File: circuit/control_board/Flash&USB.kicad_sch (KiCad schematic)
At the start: 4 parts, among them P1 USB_C_Plug_USB2.0, U13 CH440R, U14 MKDV1GCL-AB

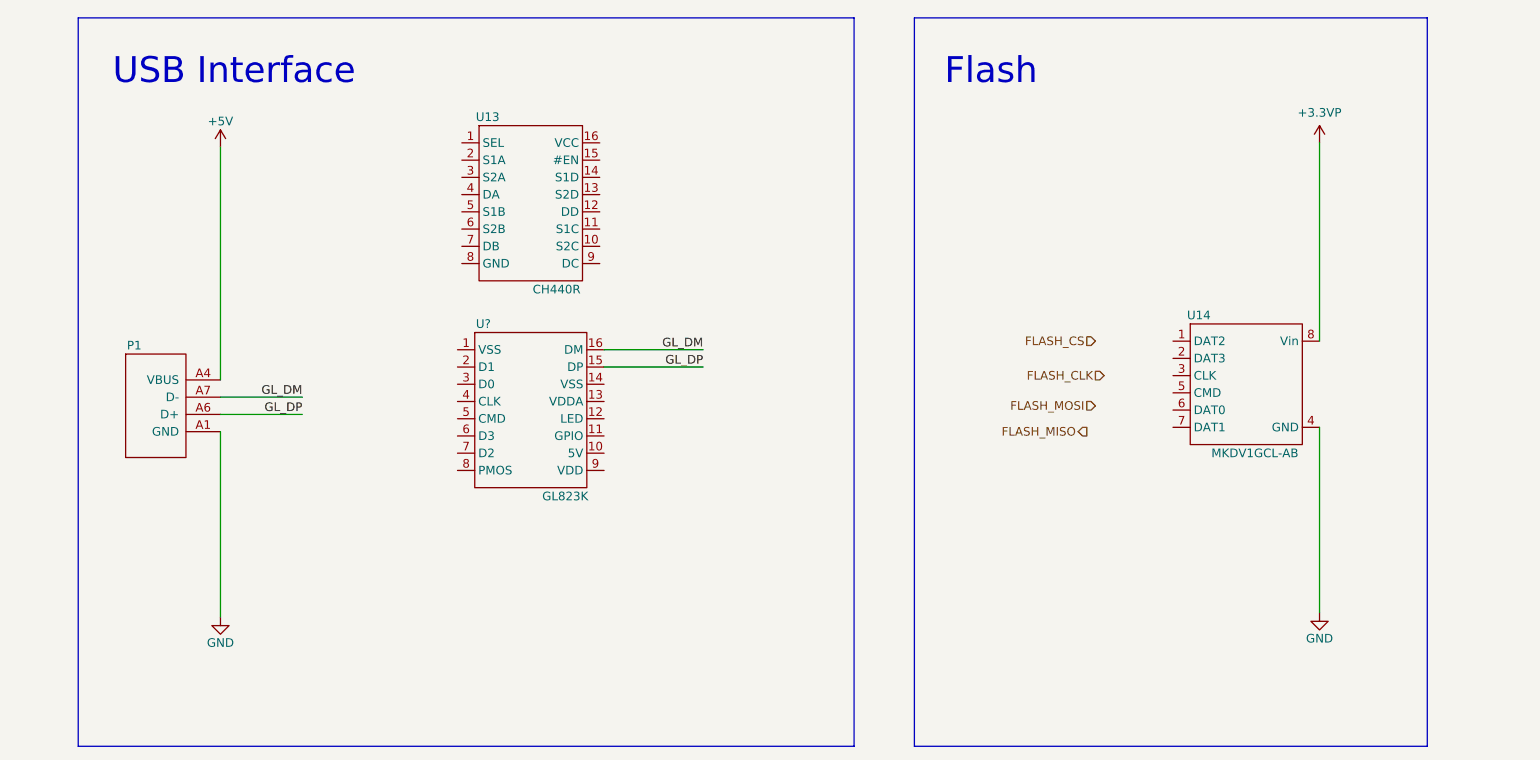
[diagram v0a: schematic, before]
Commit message: Update the main control board schematic to complete the SD card reader part.
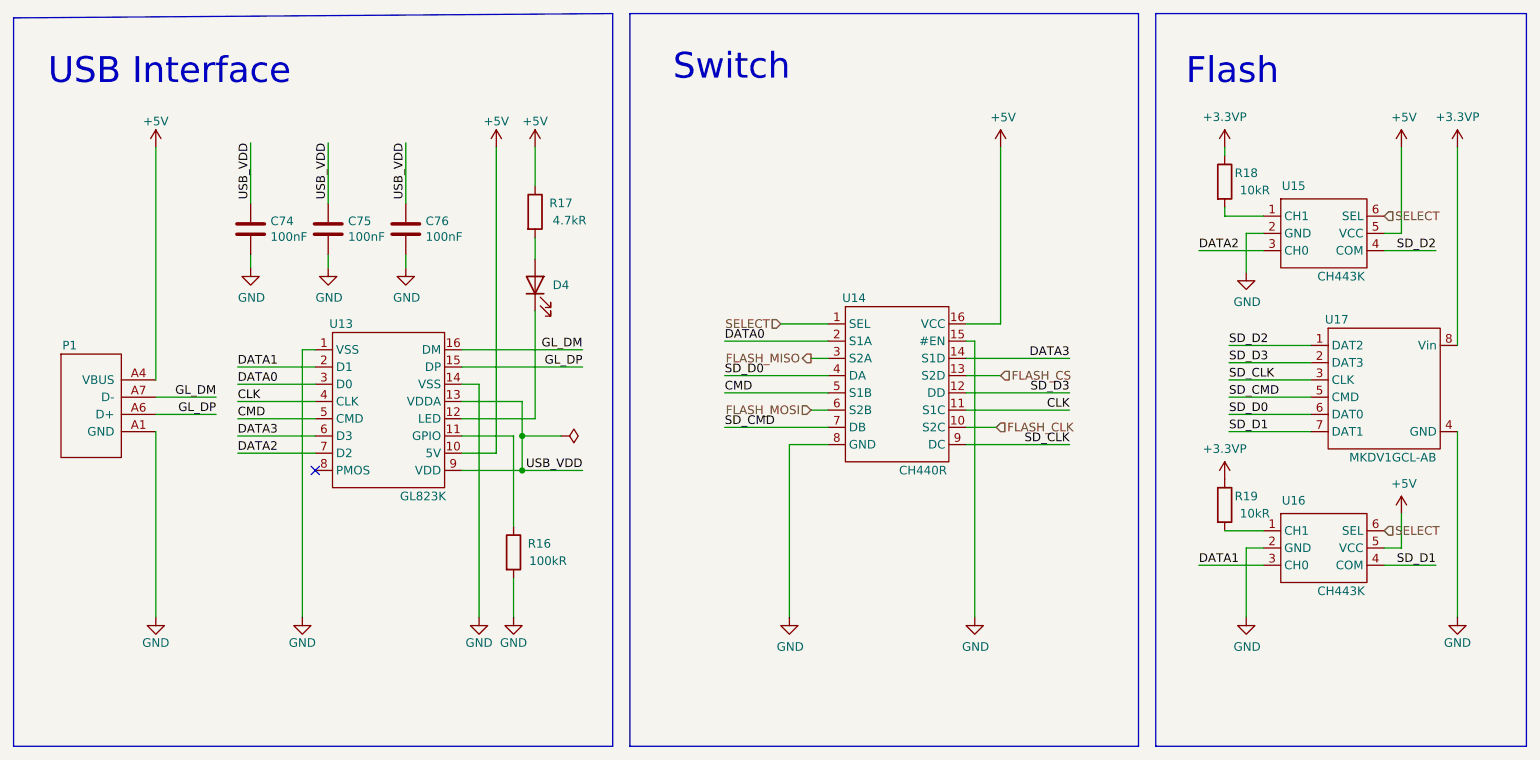
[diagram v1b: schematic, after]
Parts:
- removed U13: CH440R, ControlBoard:TSSOP-16_4.4x5mm_P0.65mm, symbol MM32_Periph:CH440R
- added C74, C75, C76: 100nF, ControlBoard:C_0603_1608Metric, symbol Device:C
- added D4: LED, ControlBoard:LED_0603_1608Metric, symbol Device:LED
- added R16: 100kR, ControlBoard:R_0603_1608Metric, symbol Device:R
- added R17: 4.7kR, ControlBoard:R_0603_1608Metric, symbol Device:R
- added R18, R19: 10kR, ControlBoard:R_0603_1608Metric, symbol Device:R
- added U14: CH440R, ControlBoard:TSSOP-16_4.4x5mm_P0.65mm, symbol MM32_Periph:CH440R
- added U15, U16: CH443K, Package_TO_SOT_SMD:SOT-363_SC-70-6, symbol MM32_Periph:CH443K
- U13: renamed from U?; footprint (none) -> Package_SO:SSOP-16_3.9x4.9mm_P0.635mm
- renumbered U14 to U17
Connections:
- net +3.3VP: now also R18.1, R19.1
- net +5V: now also U13.10 (5V), R17.1, U14.16 (VCC), U15.5 (VCC), U16.5 (VCC)
- net FLASH_CLK: now also U14.10 (S2C)
- net FLASH_CS: now also U14.13 (S2D)
- net FLASH_MISO: now also U14.3 (S2A)
- net FLASH_MOSI: now also U14.6 (S2B)
- net GND: now also U13.1 (VSS), U13.14 (VSS), C74.2, C75.2, C76.2, R16.2, U14.15 (#EN), U14.8 (GND), U15.2 (GND), U16.2 (GND)
- net at U13.11 (GPIO): now also R16.1
- net at U13.12 (LED): now also D4.1 (K)
- net USB_VDD: now reaches U13.13 (VDDA)
- net USB_VDD: now also U13.9 (VDD), C74.1, C75.1, C76.1
- net DATA1: now reaches U13.2 (D1)
- net DATA1: now also U16.3 (CH0)
- net DATA0: now reaches U13.3 (D0)
- net DATA0: now also U14.2 (S1A)
- net CLK: now reaches U13.4 (CLK)
- net CLK: now also U14.11 (S1C)
- net CMD: now reaches U13.5 (CMD)
- net CMD: now also U14.5 (S1B)
- net DATA3: now reaches U13.6 (D3)
- net DATA3: now also U14.14 (S1D)
- net DATA2: now reaches U13.7 (D2)
- net DATA2: now also U15.3 (CH0)
- net SD_D2: now reaches U17.1 (DAT2)
- net SD_D2: now also U15.4 (COM)
- net SD_D3: now reaches U17.2 (DAT3)
- net SD_D3: now also U14.12 (DD)
- net SD_CLK: now reaches U17.3 (CLK)
- net SD_CLK: now also U14.9 (DC)
- net SD_CMD: now reaches U17.5 (CMD)
- net SD_CMD: now also U14.7 (DB)
- net SD_D0: now reaches U17.6 (DAT0)
- net SD_D0: now also U14.4 (DA)
- net SD_D1: now reaches U17.7 (DAT1)
- net SD_D1: now also U16.4 (COM)
- new net: R18.2, U15.1 (CH1)
- new net: D4.2 (A), R17.2
- new net: R19.2, U16.1 (CH1)
- new net SELECT: U14.1 (SEL), U15.6 (SEL), U16.6 (SEL)
- no-connect marks 0 -> 1
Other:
- note added: "Switch"
- moved on the sheet: P1, U13, U17
